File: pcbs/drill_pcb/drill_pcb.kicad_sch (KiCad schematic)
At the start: 9 parts, among them U101 TXS0108EPW, U102 ESP32-DevKitC

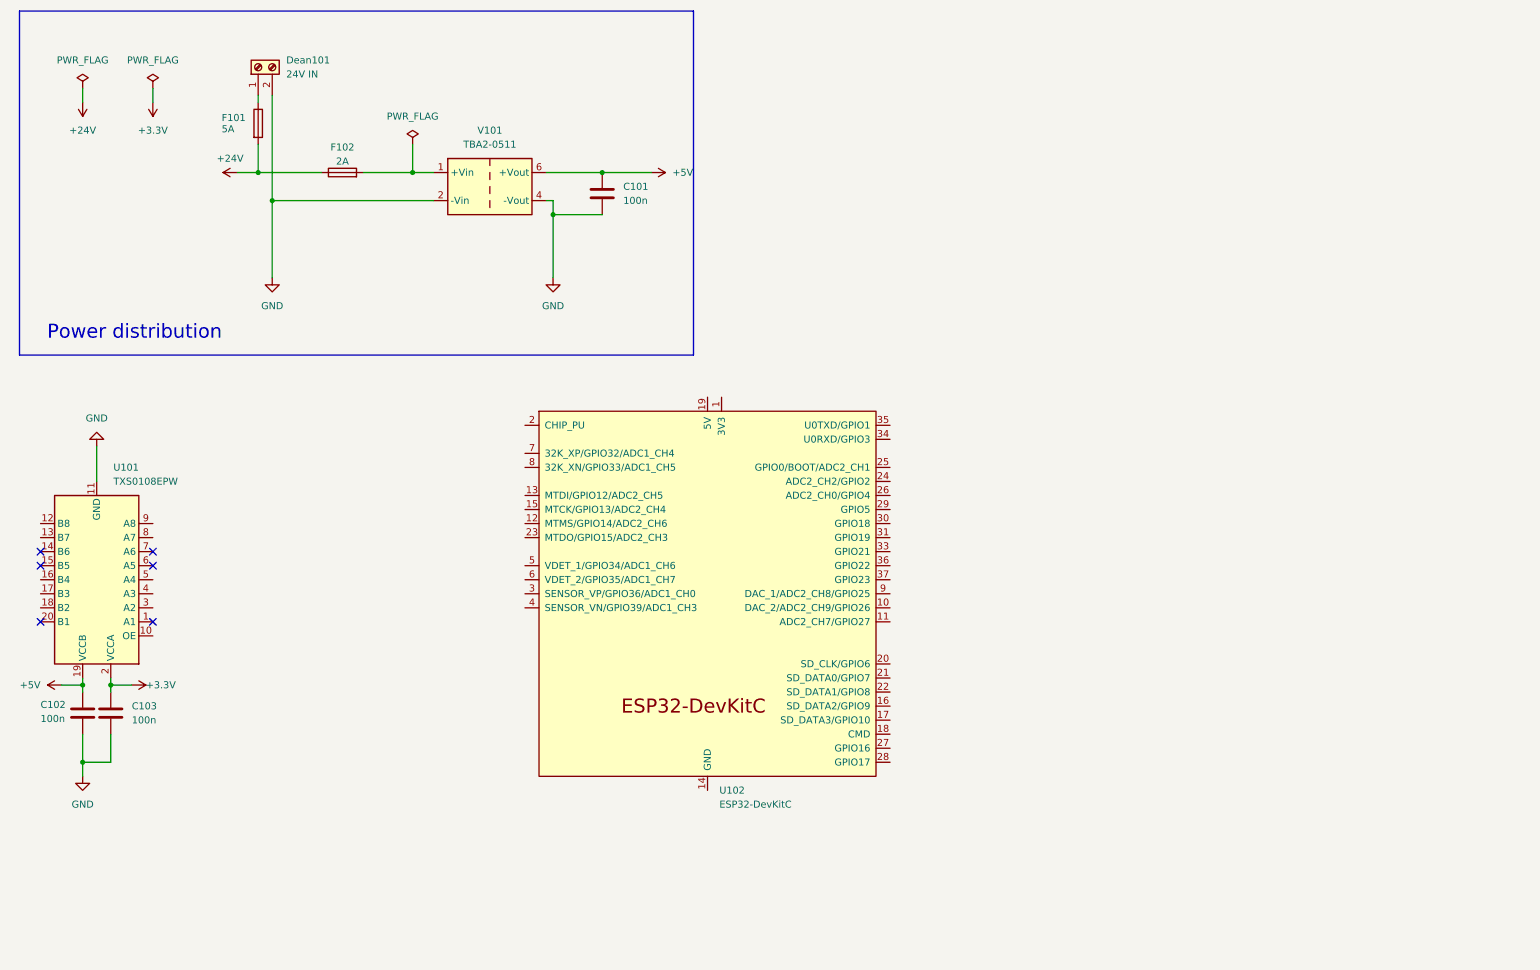
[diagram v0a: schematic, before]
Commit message: PCB changes
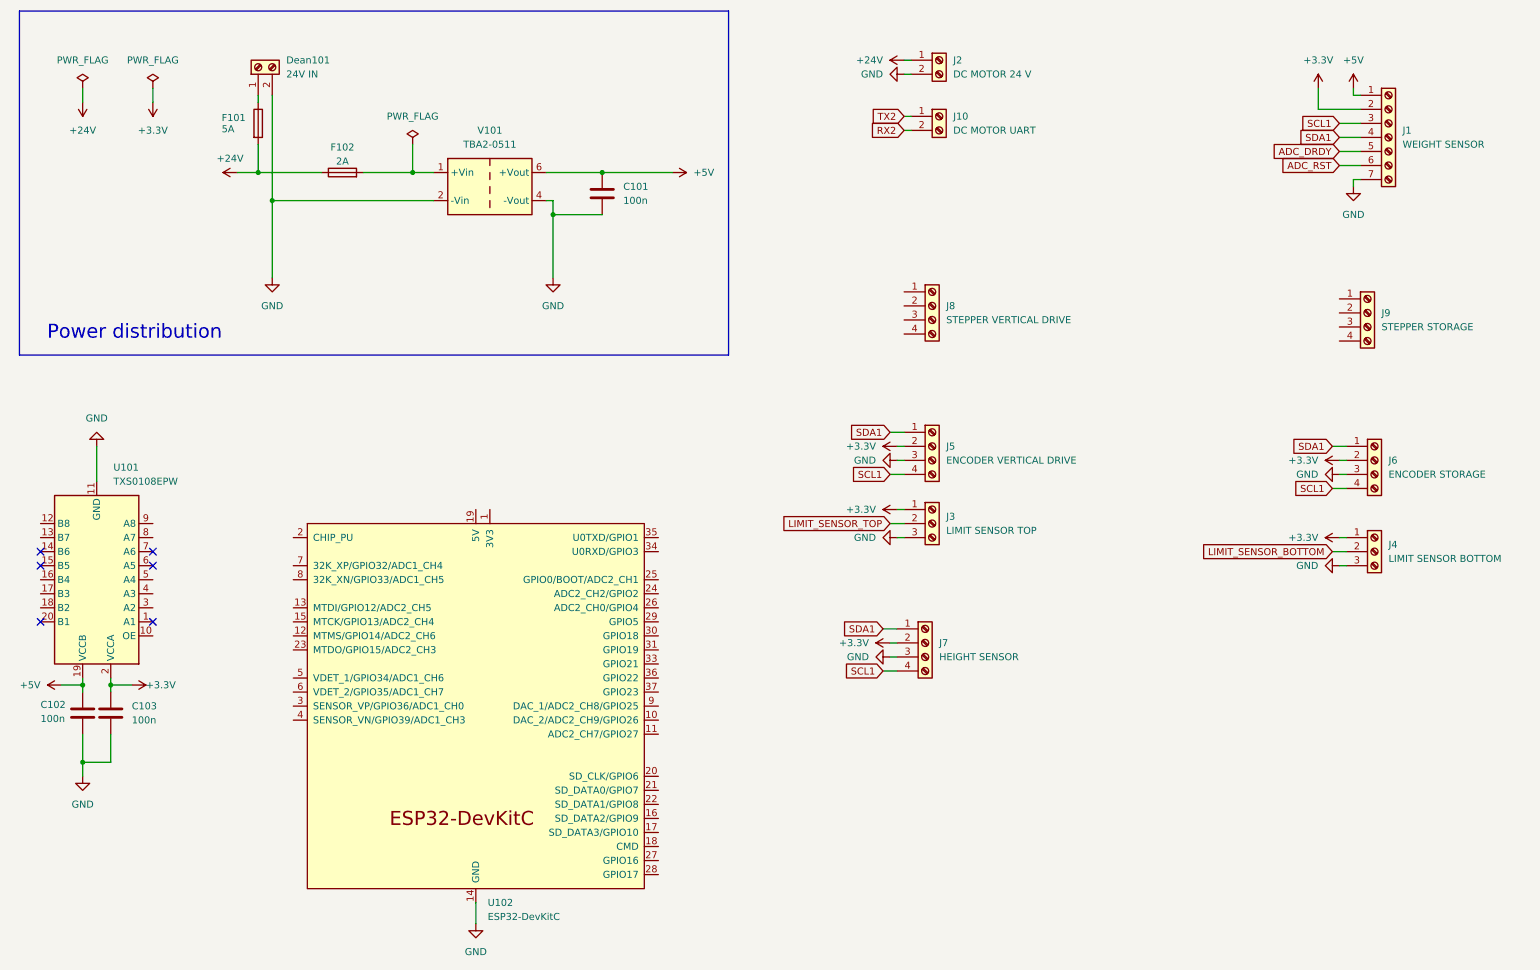
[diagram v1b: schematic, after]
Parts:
- added J1: WEIGHT SENSOR, Connector_JST:JST_XH_B7B-XH-A_1x07_P2.50mm_Vertical, symbol Connector:Screw_Terminal_01x07
- added J10: DC MOTOR UART, drill_T-DEAN:DEANS, symbol Connector:Screw_Terminal_01x02
- added J2: DC MOTOR 24 V, drill_T-DEAN:DEANS, symbol Connector:Screw_Terminal_01x02
- added J3: LIMIT SENSOR TOP, Connector_JST:JST_XH_B3B-XH-A_1x03_P2.50mm_Vertical, symbol Connector:Screw_Terminal_01x03
- added J4: LIMIT SENSOR BOTTOM, Connector_JST:JST_XH_B3B-XH-A_1x03_P2.50mm_Vertical, symbol Connector:Screw_Terminal_01x03
- added J5: ENCODER VERTICAL DRIVE, Connector_JST:JST_XH_B4B-XH-A_1x04_P2.50mm_Vertical, symbol Connector:Screw_Terminal_01x04
- added J6: ENCODER STORAGE, Connector_JST:JST_XH_B4B-XH-A_1x04_P2.50mm_Vertical, symbol Connector:Screw_Terminal_01x04
- added J7: HEIGHT SENSOR, Connector_JST:JST_XH_B4B-XH-A_1x04_P2.50mm_Vertical, symbol Connector:Screw_Terminal_01x04
- added J8: STEPPER VERTICAL DRIVE, Connector_JST:JST_XH_B4B-XH-A_1x04_P2.50mm_Vertical, symbol Connector:Screw_Terminal_01x04
- added J9: STEPPER STORAGE, Connector_JST:JST_XH_B4B-XH-A_1x04_P2.50mm_Vertical, symbol Connector:Screw_Terminal_01x04
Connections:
- net +24V: now also J2.1 (Pin_1)
- net +3.3V: now also J1.2 (Pin_2), J3.1 (Pin_1), J4.1 (Pin_1), J5.2 (Pin_2), J6.2 (Pin_2), J7.2 (Pin_2)
- net +5V: now also J1.1 (Pin_1)
- net GND: now also U102.14 (GND), U102.32 (GND), U102.38 (GND), J1.7 (Pin_7), J2.2 (Pin_2), J3.3 (Pin_3), J4.3 (Pin_3), J5.3 (Pin_3), J6.3 (Pin_3), J7.3 (Pin_3)
- new net ADC_DRDY: J1.5 (Pin_5)
- new net ADC_RST: J1.6 (Pin_6)
- new net LIMIT_SENSOR_BOTTOM: J4.2 (Pin_2)
- new net LIMIT_SENSOR_TOP: J3.2 (Pin_2)
- new net RX2: J10.2 (Pin_2)
- new net SCL1: J1.3 (Pin_3), J5.4 (Pin_4), J6.4 (Pin_4), J7.4 (Pin_4)
- new net SDA1: J1.4 (Pin_4), J5.1 (Pin_1), J6.1 (Pin_1), J7.1 (Pin_1)
- new net TX2: J10.1 (Pin_1)
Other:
- moved on the sheet: U102
